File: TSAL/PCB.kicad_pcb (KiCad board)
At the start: 4 copper layers, 100 x 50 mm, 63 parts, among them J1 TE 770966-2, J2 JST B04B-XASK, J3 Conn_01x02, J4 Conn_01x02, Q1 IRLZ44N, Q2 MMBT3904, Q3 IRLZ44N, U1 TL431D, U2 LMV331, U3 UCC12040DVE, U4 LTV-817S, U5 LM555xN, U7 MP174AGJ-Z

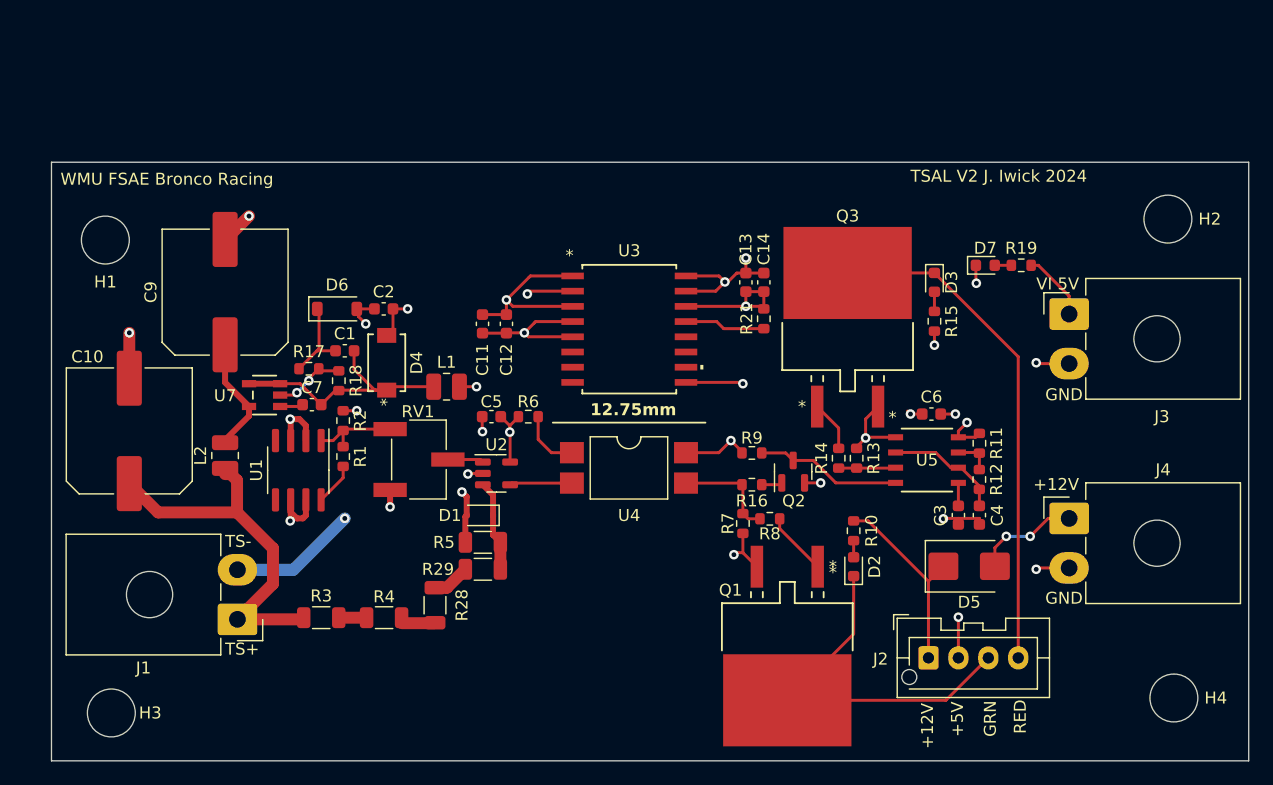
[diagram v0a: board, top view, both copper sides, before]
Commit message: TSAL REV3 :(
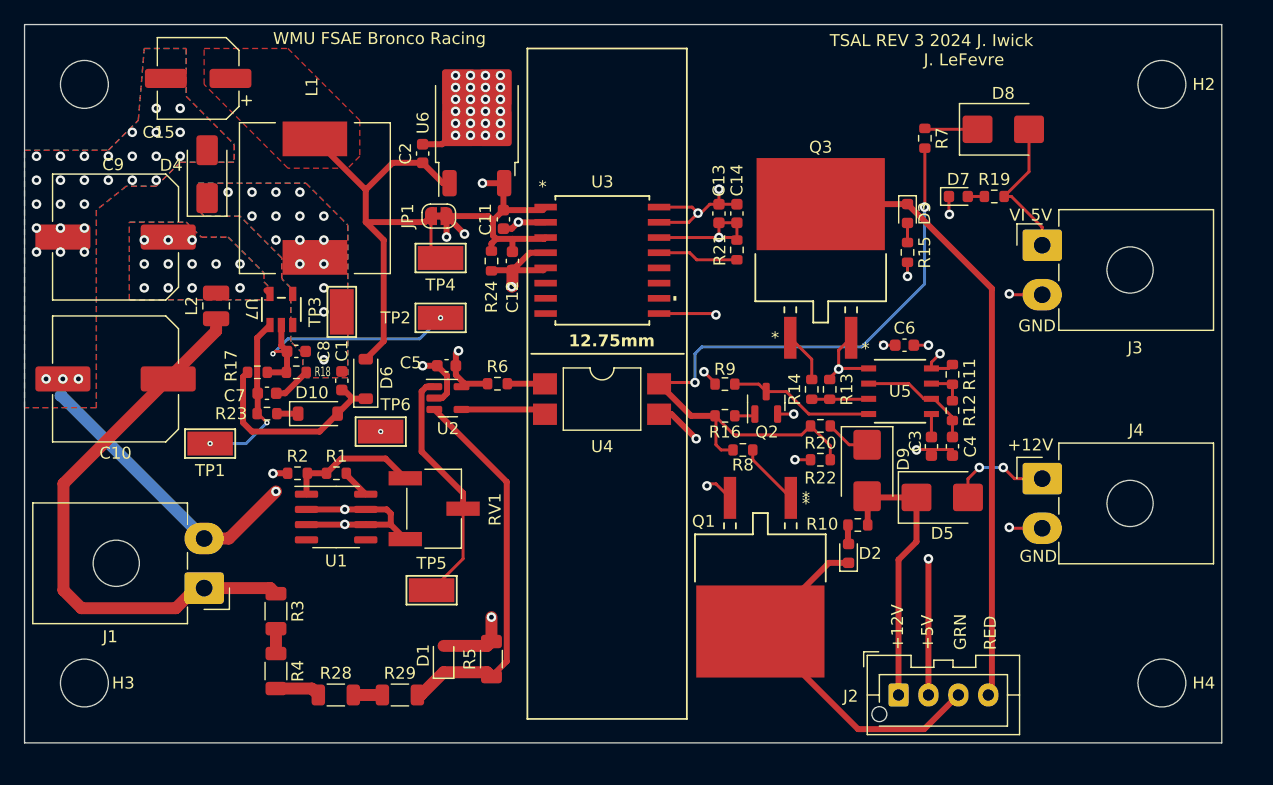
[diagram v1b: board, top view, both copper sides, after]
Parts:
- added C15: 100u, Capacitor_SMD:CP_Elec_6.3x7.7, F.Cu at (114.5, 79.5)
- added C8: 470p, Capacitor_SMD:C_0603_1608Metric, F.Cu at (122.7, 102.3)
- added D10: 1N4148WS, Diode_SMD:D_SOD-123, F.Cu at (124.5, 107.5)
- added D8: SSB43L, Diode_SMD:D_SMB, F.Cu at (181.8, 83.8)
- added D9: SSB43L, Diode_SMD:D_SMB, F.Cu at (170.4, 112.2)
- added JP1: SolderJumper_2_Bridged, Jumper:SolderJumper-2_P1.3mm_Bridged_RoundedPad1.0x1.5mm, F.Cu at (134.6, 91.0)
- added R20: 22k, Resistor_SMD:R_0603_1608Metric, F.Cu at (166.5, 108.5)
- added R22: 220k, Resistor_SMD:R_0603_1608Metric, F.Cu at (166.5, 111.3)
- added R23: 24k, Resistor_SMD:R_0603_1608Metric, F.Cu at (120.2, 107.5)
- added R24: 1k, Resistor_SMD:R_0603_1608Metric, F.Cu at (139.0, 94.8)
- added TP1: TestPoint, TestPoint:TestPoint_Keystone_5019_Minature, F.Cu at (115.5, 110.0)
- added TP2: TestPoint, TestPoint:TestPoint_Keystone_5019_Minature, F.Cu at (134.8, 99.5)
- added TP3: TestPoint, TestPoint:TestPoint_Keystone_5019_Minature, F.Cu at (126.5, 99.0)
- added TP4: TestPoint, TestPoint:TestPoint_Keystone_5019_Minature, F.Cu at (134.8, 94.5)
- added TP5: TestPoint, TestPoint:TestPoint_Keystone_5019_Minature, F.Cu at (134.0, 122.2)
- added TP6: TestPoint, TestPoint:TestPoint_Keystone_5019_Minature, F.Cu at (129.8, 109.0)
- added U6: LF50_TO252, Package_TO_SOT_SMD:TO-252-2, F.Cu at (137.8, 83.2)
- C1: value 100n -> 220n
- C2: value 100u -> 0.1u
- D4: value AES2JF-HF -> STTH1R06A; footprint KiCADv6:CR_SMAF_CIP -> Diode_SMD:D_SMA
- L1: footprint Inductor_SMD:L_1008_2520Metric -> Inductor_SMD:L_12x12mm_H8mm
- R16: value 22k -> 220k
- R17, R18: value 5k -> 20k
- R6: value 2.2k -> 1k
- R7: value 100k -> 10k
- moved R7 35.6 mm to (175.2, 84.5)
- moved D4 21.8 mm to (115.2, 87.5)
- moved L1 19.2 mm to (124.2, 89.5), turned to 90 degrees
- moved C2 13.4 mm to (133.2, 85.8), turned to 90 degrees
- moved H1 13.1 mm to (105.0, 80.0)
- moved R29 12.6 mm to (131.4, 131.0)
- moved L2 12.5 mm to (116.0, 98.5)
- moved D1 12.4 mm to (135.0, 128.0), turned to 90 degrees
- moved H2 11.3 mm to (195.0, 80.0)
- moved R28 11.2 mm to (126.0, 131.0), turned to 0 degrees
- moved C9 10.2 mm to (107.6, 92.8), turned to 180 degrees
- moved R4 10.1 mm to (121.0, 129.0), turned to -90 degrees
- moved R5 9.78 mm to (139.0, 128.0), turned to 90 degrees
- moved C11 8.90 mm to (140.0, 91.3)
- moved U2 7.49 mm to (135.4, 106.2)
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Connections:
- C2 pad 1: +5V -> Net-(D6-A)
- D6 pad 2: +5V -> Net-(D6-A)
- L1 pad 2: +5V -> Net-(D6-A)
- R7 pad 1: Net-(R16-Pad1) -> Net-(D8-K)
- R7 pad 2: GND -> Net-(R16-Pad1)
- U4 pad 3: Net-(R16-Pad1) -> GND
- U4 pad 4: +5V@GLV -> Net-(R16-Pad1)
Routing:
- net Net-(R16-Pad1): track 8.89 -> 61.0 mm, vias 0 -> 2
- net Net-(D6-A): track 0.00 -> 41.5 mm
- net Net-(D1-K): track 7.66 -> 32.5 mm
- net Net-(D4-K): track 21.8 -> 3.22 mm, vias 0 -> 16
- net Net-(U2-+): track 3.01 -> 20.4 mm
- net Net-(U7-FB): track 5.74 -> 22.2 mm
- net TS+: track 30.9 -> 46.7 mm
- net TS-: track 55.9 -> 69.5 mm, vias 12 -> 62
- net Net-(U7-VCC): track 1.94 -> 14.5 mm, vias 0 -> 2
- net +5V@GLV: track 31.7 -> 42.0 mm
- net Net-(D10-A): track 7.24 -> 17.3 mm
- net Net-(U7-DRAIN): track 9.46 -> 0.42 mm, vias 0 -> 12
- net /Ext-LED-RED: track 42.3 -> 51.3 mm
- net +12V: track 16.5 -> 23.8 mm
- net +5V: track 25.9 -> 31.6 mm
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- added copper zone on B.Cu, net Net-(D4-K)
- added copper zone on F.Cu, net Net-(D4-K)
- added copper zone on In1.Cu, net Net-(D4-K)
- added copper zone on In2.Cu, net Net-(D4-K)
- added copper zone on F.Cu, net Net-(D6-A)
- added copper zone on B.Cu, net Net-(U7-DRAIN)
- added copper zone on F.Cu, net Net-(U7-DRAIN)
- added copper zone on In1.Cu, net Net-(U7-DRAIN)
- added copper zone on In2.Cu, net Net-(U7-DRAIN)
- added copper zone on B.Cu, net TS-
- added copper zone on F.Cu, net TS-
- added copper zone on In2.Cu, net TS-
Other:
- board size 100 x 50 mm -> 100 x 60 mm
- board text added: "Bronco Racing TSAL + Voltage Indicator REV 3"
- board text added: "TSAL REV 3 2024 J. Iwick J. LeFevre"
- board text removed: "Bronco Racing TSAL + Voltage Indicator Rev 2"
- board text removed: "Josh Iwick Feb 2023"
- board text removed: "TS+"
- board text removed: "TS-"
- board text removed: "TSAL V2 J. Iwick 2024"
